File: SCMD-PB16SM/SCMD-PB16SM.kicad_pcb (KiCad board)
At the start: 2 copper layers, 200 x 100 mm, 68 parts, among them J1 Logic Supply, M1 SCMD, M10 SCMD, M11 SCMD, M12 SCMD, M2 SCMD, M3 SCMD, M4 SCMD, M5 SCMD, M6 SCMD, M7 SCMD, M8 SCMD, M9 SCMD

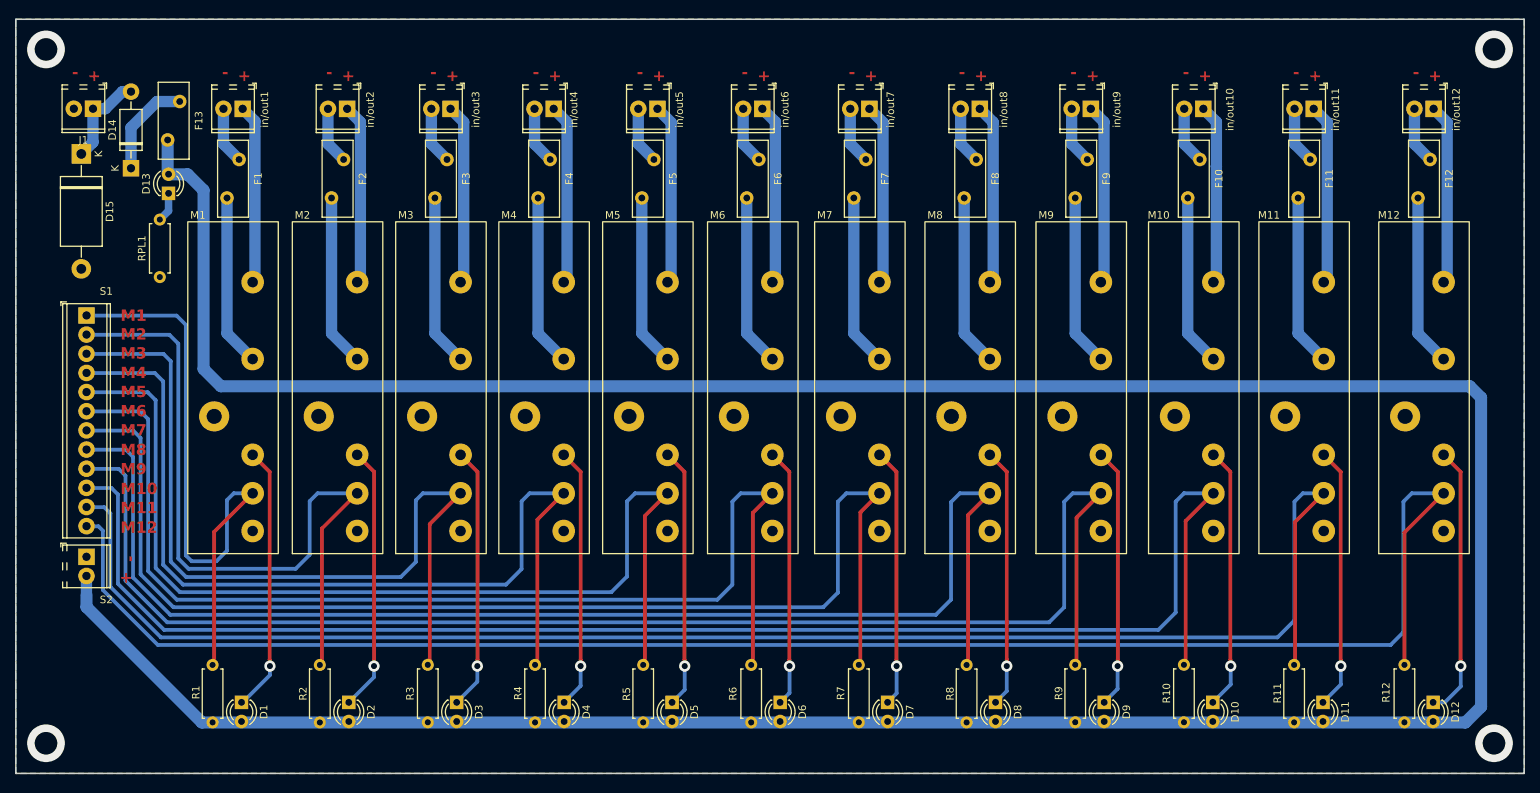
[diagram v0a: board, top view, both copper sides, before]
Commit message: Add files via upload
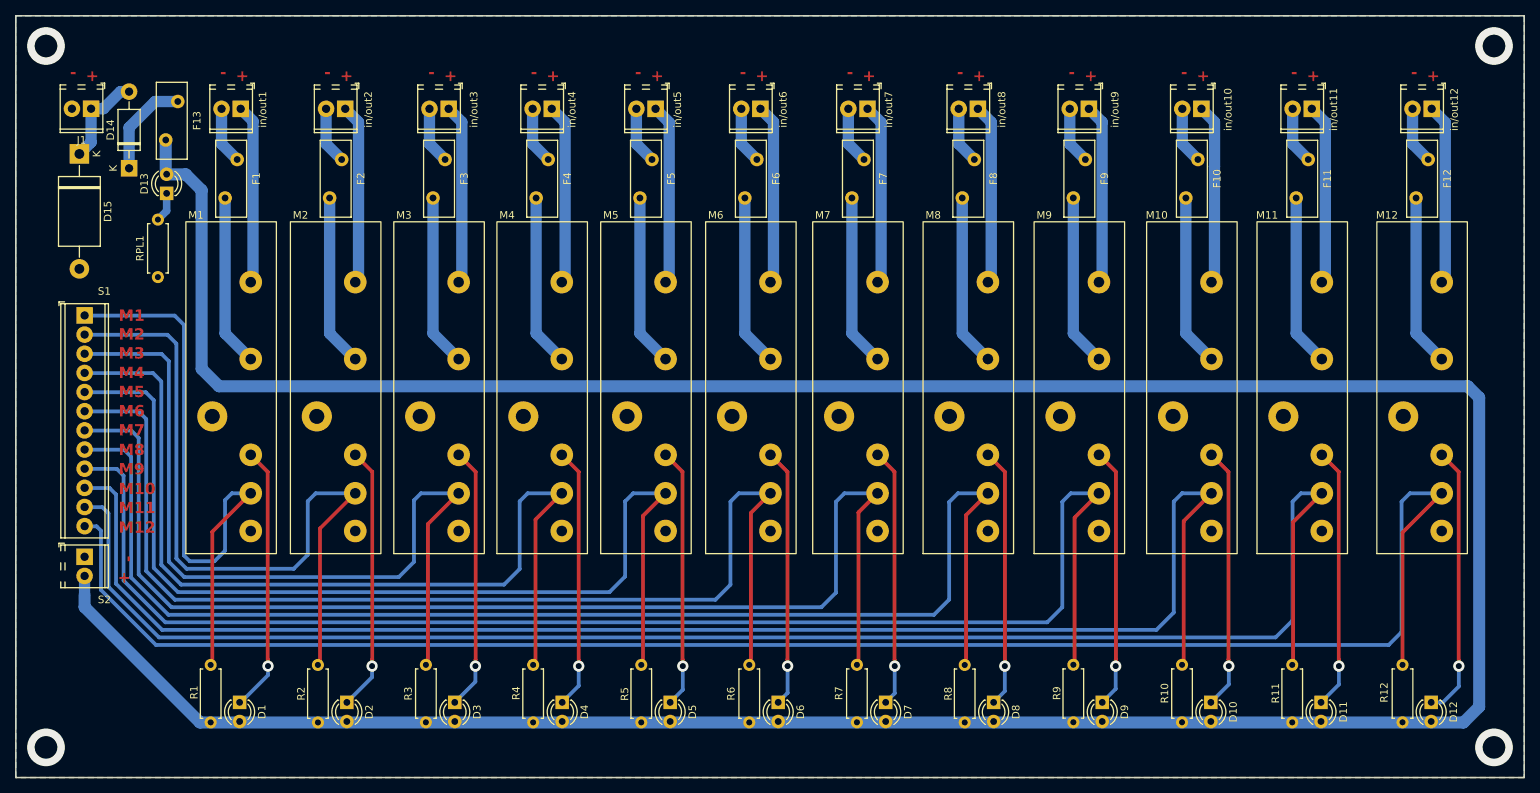
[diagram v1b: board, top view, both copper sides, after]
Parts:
- moved D10 0.25 mm to (184.5, 107.6)
- moved D11 0.25 mm to (199.1, 107.6)
- moved D12 0.25 mm to (213.7, 107.6)
- moved D13 0.25 mm to (46.0, 40.1)
- moved D14 0.25 mm to (41.0, 36.8)
- moved D15 0.25 mm to (34.4, 34.9)
- moved D2 0.25 mm to (69.9, 107.6)
- moved D3 0.25 mm to (84.2, 107.6)
- moved D5 0.25 mm to (112.8, 107.6)
- moved D6 0.25 mm to (127.1, 107.6)
- moved D7 0.25 mm to (141.3, 107.6)
- moved D8 0.25 mm to (155.7, 107.6)
- moved D9 0.25 mm to (170.1, 107.6)
- moved F1 0.25 mm to (55.3, 35.6)
- moved F10 0.25 mm to (182.7, 35.6)
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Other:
- board size 200 x 100 mm -> 200 x 101 mm
